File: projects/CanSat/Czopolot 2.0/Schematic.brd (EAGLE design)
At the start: 43 x 30.8 mm, 91 parts

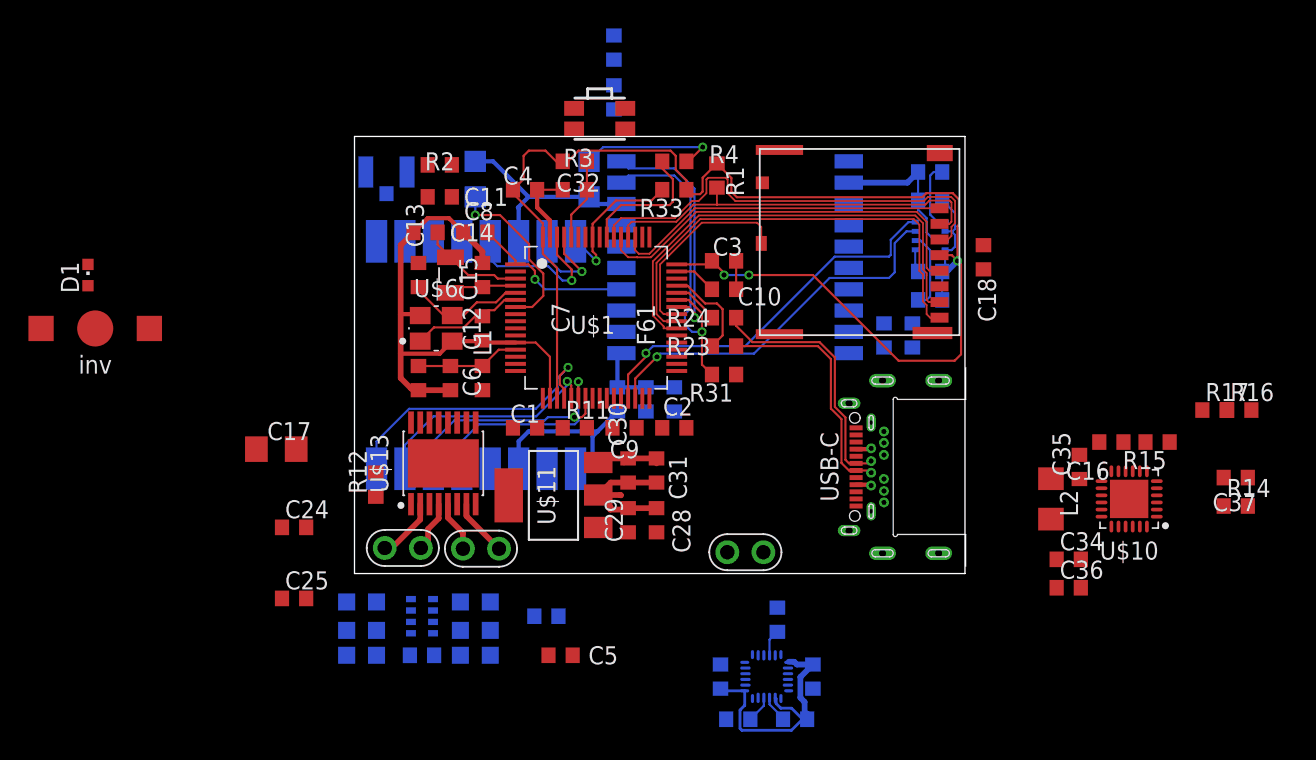
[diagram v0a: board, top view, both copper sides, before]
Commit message: Work work..
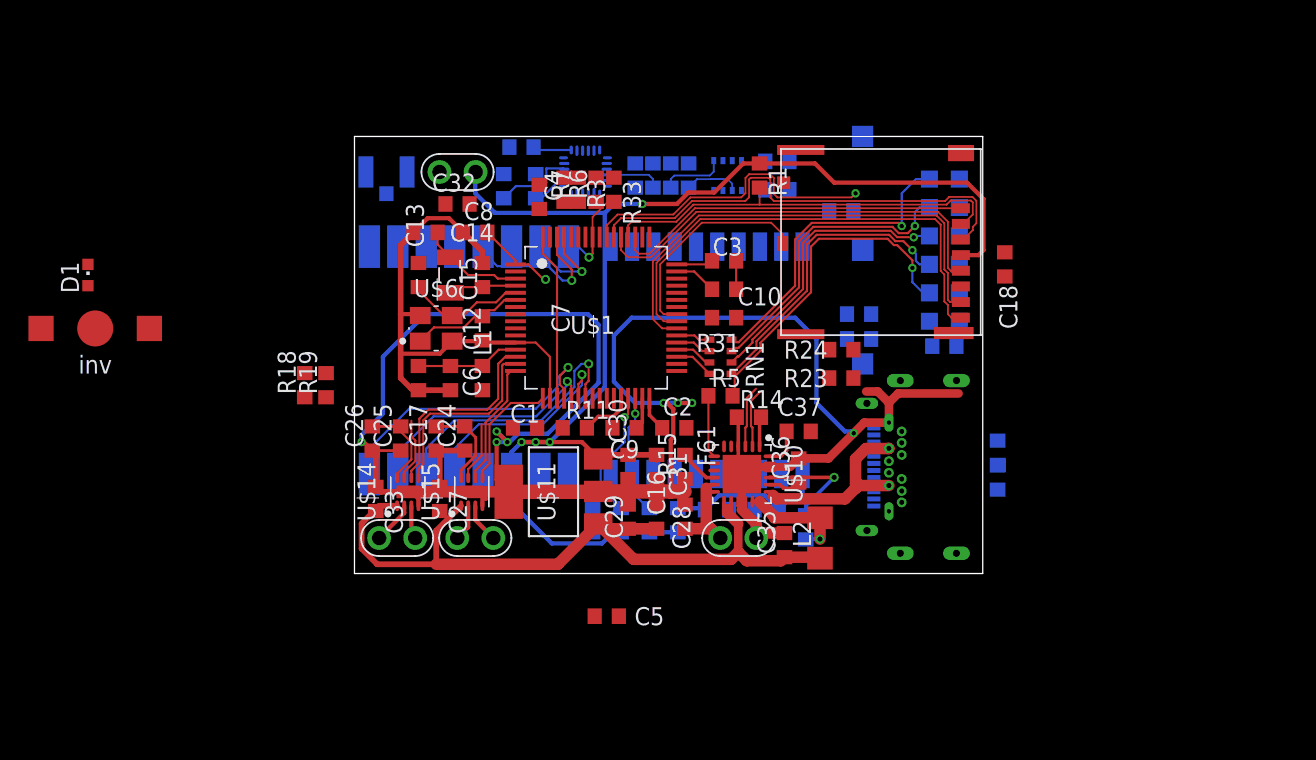
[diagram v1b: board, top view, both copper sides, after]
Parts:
- removed U$13: DRV8833SOP, SobieskiSat2:SOP65P640X120-17T340X500N
- added C26: 10u, Unified:C0603
- added C27, C33: 100n, Unified:C0603
- added R18, R19: 100k, Unified:R0603
- added U$14, U$15: DRV8838, SobieskiSat2:SON50P200X200X80-9T90X160N
- BTN_DFU: value PUSH-SWITCH -> PUSH-SWITCHDIP; device SobieskiSat2:SWITCH_SMD -> SobieskiSat2:2X1_2.54
- C17: value 10u_pol -> 100n; device Unified:C1206 -> Unified:C0603
- C24: value 100n -> 10u
- C25: value 2.2u -> 100n
- R12: value 10k -> 100k
- moved D7 50.7 mm to (39.2, 25.8), turned to 90 degrees
- moved D8 48.4 mm to (39.2, 23.8), turned to 90 degrees
- moved D10 47.3 mm to (39.2, 17.8)
- moved D6 45.8 mm to (39.2, 27.8)
- moved R30 42.7 mm to (39.2, 16.0), turned to 180 degrees
- moved D2 41.7 mm to (39.2, 19.8)
- moved C21 41.0 mm to (8.25, 27.2), turned to 270 degrees
- moved D9 40.7 mm to (39.2, 21.8)
- moved R10 39.9 mm to (17.5, 28.0), turned to 90 degrees
- moved C23 39.8 mm to (9.50, 30.0), turned to 0 degrees
- moved C22 39.6 mm to (10.5, 27.2), turned to 90 degrees
- moved U$9 37.7 mm to (14.0, 28.2), turned to 90 degrees
- moved R14 34.8 mm to (25.5, 11.0)
- moved R15 33.3 mm to (21.0, 7.50), turned to 90 degrees
- moved D61 33.3 mm to (14.5, 3.75)
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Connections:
- removed net AIN1: U$13.16
- removed net AIN2: U$13.15
- removed net BIN1: U$13.9
- removed net BIN2: U$13.10
- removed net N$51: D10.A, R30.2
- new net EN_L: U$1.15, U$14.5
- new net EN_R: U$1.17, U$15.5
- new net N$32: D10.C, R30.1
- new net N$33: D61.1, R63.1, U$3.P$10
- new net N$34: MOTR.P$2, U$15.2
- new net N$36: MOTR.P$1, U$15.3
- new net N$39: C17.2, C24.2, U$15.8
- new net N$40: R19.1, U$15.7
- new net PH_L: U$1.14, U$14.6
- new net PH_R: U$1.16, U$15.6
- net DFU: no longer BTN_DFU.P$3
- net GND: now also C17.1, C24.1, C26.1, C27.1, C33.1, R30.2, U$14.4, U$14.9, U$15.4, U$15.9; no longer D10.C, U$13.13, U$13.17
- net GPS_RX: now also D61.2, U$1.29; no longer U$1.42, U$3.P$10
- net GPS_TX: now also R12.2, U$1.30; no longer R31.2, U$1.43
- net N$10: now also R5.1, U$10.7; no longer MOTL.P$2, U$13.2
- net N$15: now also RN1.1, U$1.38; no longer MOTR.P$1, U$13.5
- net N$19: now also RN1.2, U$1.37; no longer C17.1, C24.1, U$13.11
- net N$20: now also RN1.3, U$1.36; no longer D2.C, U$10.7
- net N$26: now also MOTL.P$1, U$14.3; no longer C25.2, U$13.14
- net N$28: now also RN1.4, U$1.35; no longer D2.A, R5.1
- net N$29: now also R31.2, U$1.43; no longer U$13.3
- net N$3: now also D2.C, R5.2; no longer MOTR.P$2, U$13.7
- net N$30: now also C25.2, C26.2, U$14.8; no longer U$13.6
- net N$31: now also R18.1, U$14.7; no longer R12.1, U$13.1
- net N$5: now also MOTL.P$2, U$14.2; no longer MOTL.P$1, U$13.4
- net SCL: now also R6.1, U$1.58; no longer R7.2, U$1.29
- net SDA: now also R7.1, U$1.59; no longer R6.2, U$1.30
- net VCC: now also D10.A, D2.A, R12.1, R18.2, R19.2, R6.2, R63.2, R7.2; no longer BTN_DFU.P$4, R12.2, R30.1, R5.2, R6.1, R7.1
- net VSYS: now also C27.2, C33.2, U$14.1, U$15.1; no longer C17.2, C24.2, U$13.12
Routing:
- net GND: track 84.0 -> 193.7 mm, vias 0 -> 8
- net VSYS: track 0.00 -> 54.0 mm
- net SCL: track 27.1 -> 0.00 mm, vias 1 -> 0
- net SDA: track 26.6 -> 0.00 mm, vias 1 -> 0
- net N$38: track 0.00 -> 22.2 mm, vias 0 -> 1
- net N$1: track 0.00 -> 21.4 mm, vias 0 -> 1
- net N$37: track 0.00 -> 21.0 mm, vias 0 -> 1
- net VCC: track 138.4 -> 117.7 mm, vias 3 -> 4
- net N$2: track 0.00 -> 20.0 mm, vias 0 -> 1
- net N$3: track 4.08 -> 23.8 mm, vias 0 -> 1
- net GPS_TX: track 23.2 -> 8.61 mm
- net PH_L: track 0.00 -> 14.4 mm
- net EN_L: track 0.00 -> 13.8 mm
- net USB_D-: track 17.9 -> 4.37 mm
- net USB_D+: track 17.0 -> 4.10 mm
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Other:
- board size 43 x 30.8 mm -> 44.2 x 30.8 mm
- board text removed: "^ Battery and switch holes or pads"
